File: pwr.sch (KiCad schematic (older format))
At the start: 12 parts, among them J6 Conn_01x02, Q2 FDC6420C, U5 SGM2036_UTDFN, U7 SGM40561

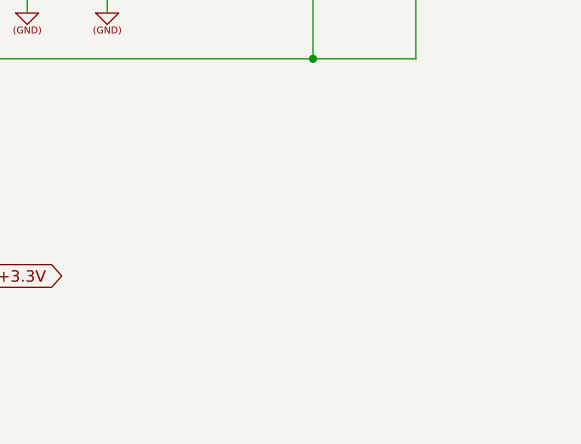
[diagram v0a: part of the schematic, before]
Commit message: Build power board
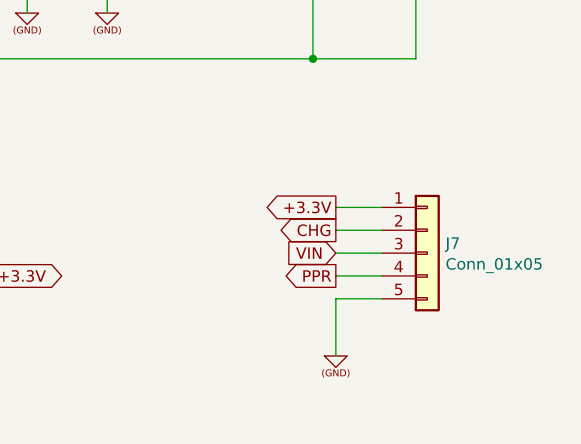
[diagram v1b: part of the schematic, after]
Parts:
- added J7: Conn_01x05, Pin_Headers:Pin_Header_Straight_1x05_Pitch2.54mm, symbol Connector_Generic:Conn_01x05
- Q2: footprint TO_SOT_Packages_SMD:SOT-666 -> TO_SOT_Packages_SMD:SuperSOT-6
- U5: footprint (none) -> TO_SOT_Packages_SMD:SOT-23-5
- U7: footprint Housings_DFN_QFN:VDFN-8-1EP_2x2mm_Pitch0.5mm -> Housings_DFN_QFN:TDFN-2x2-8L
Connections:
- wire segments 56 -> 62
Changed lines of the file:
@@
 F 0 "U7" H 4350 4600 50  0000 C CNN
 F 1 "SGM40561" H 5050 4550 50  0000 C CNN
-F 2 "Housings_DFN_QFN:VDFN-8-1EP_2x2mm_Pitch0.5mm" H 4650 4100 50  0001 C CNN
+F 2 "Housings_DFN_QFN:TDFN-2x2-8L" H 4650 4100 50  0001 C CNN
 F 3 "" H 4650 4100 50  0001 C CNN
 	1    4650 4100
@@
 F 0 "U5" H 4600 6582 50  0000 C CNN
 F 1 "SGM2036_UTDFN" H 4600 6491 50  0000 C CNN
-F 2 "" H 4600 6050 50  0001 C CNN
+F 2 "TO_SOT_Packages_SMD:SOT-23-5" H 4600 6050 50  0001 C CNN
 F 3 "" H 4600 6050 50  0001 C CNN
 	1    4600 6050
@@
 F 0 "Q2" V 7178 3900 50  0000 C CNN
 F 1 "FDC6420C" V 7087 3900 50  0000 C CNN
-F 2 "TO_SOT_Packages_SMD:SOT-666" H 7050 3825 50  0001 L CNN
+F 2 "TO_SOT_Packages_SMD:SuperSOT-6" H 7050 3825 50  0001 L CNN
 F 3 "http://www.irf.com/product-info/datasheets/data/irf7309ipbf.pdf" H 6850 3900 50  0001 L CNN
 	2    6850 3900
@@
 Wire Wire Line
 	4100 3100 4550 3100
+Text GLabel 6950 5650 0    50   Input ~ 0
+VIN
+$Comp
+L power:(GND) #PWR024
+U 1 1 5DA84AA6
+P 6950 6100
+F 0 "#PWR024" H 6950 6100 30  0001 C CNN
+F 1 "(GND)" H 6950 6100 30  0001 C CNN
+F 2 "" H 6950 6100 60  0000 C CNN
+F 3 "" H 6950 6100 60  0000 C CNN
+	1    6950 6100
+	1    0    0    -1
+$EndComp
+Text GLabel 6950 5450 0    50   Output ~ 0
++3.3V
+Text GLabel 6950 5550 0    50   Output ~ 0
+CHG
+Text GLabel 6950 5750 0    50   Output ~ 0
+PPR
+$Comp
+L Connector_Generic:Conn_01x05 J7
+U 1 1 5DA87273
+P 7350 5650
+F 0 "J7" H 7430 5692 50  0000 L CNN
+F 1 "Conn_01x05" H 7430 5601 50  0000 L CNN
+F 2 "Pin_Headers:Pin_Header_Straight_1x05_Pitch2.54mm" H 7350 5650 50  0001 C CNN
+F 3 "~" H 7350 5650 50  0001 C CNN
+	1    7350 5650
+	1    0    0    -1
+$EndComp
+Wire Wire Line
+	7150 5850 6950 5850
+Wire Wire Line
+	6950 5850 6950 6100
+Wire Wire Line
+	7150 5750 6950 5750
+Wire Wire Line
+	7150 5650 6950 5650
+Wire Wire Line
+	7150 5550 6950 5550
+Wire Wire Line
+	7150 5450 6950 5450
 $EndSCHEMATC

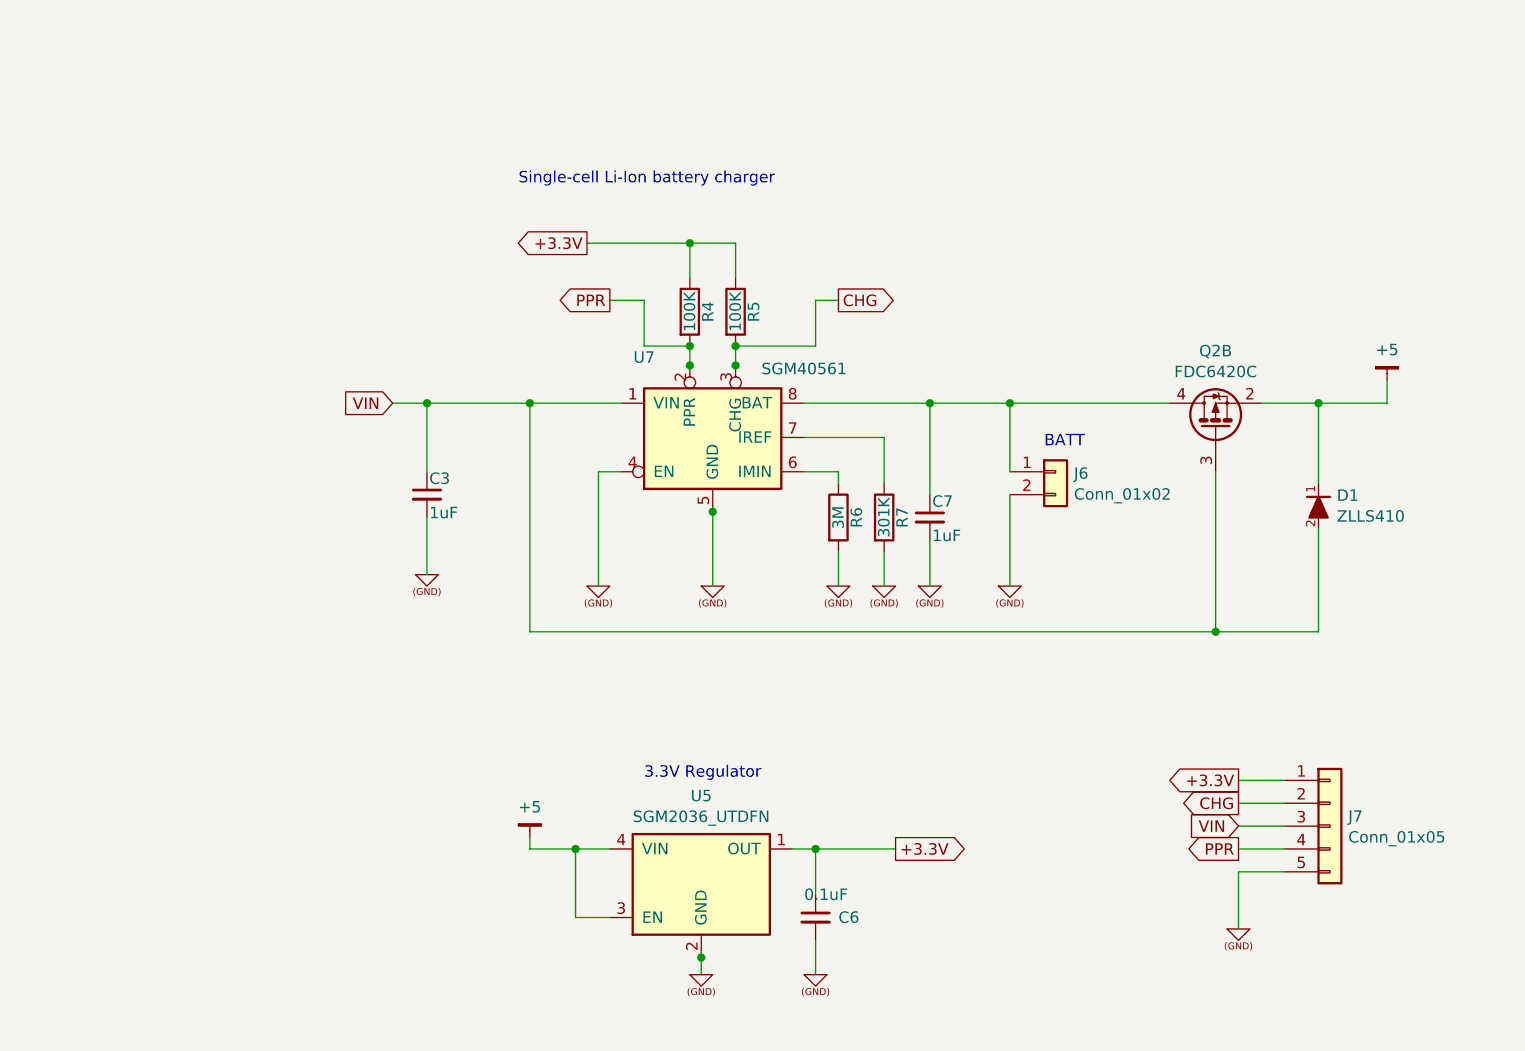
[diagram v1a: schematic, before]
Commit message: v.01 power board PCB
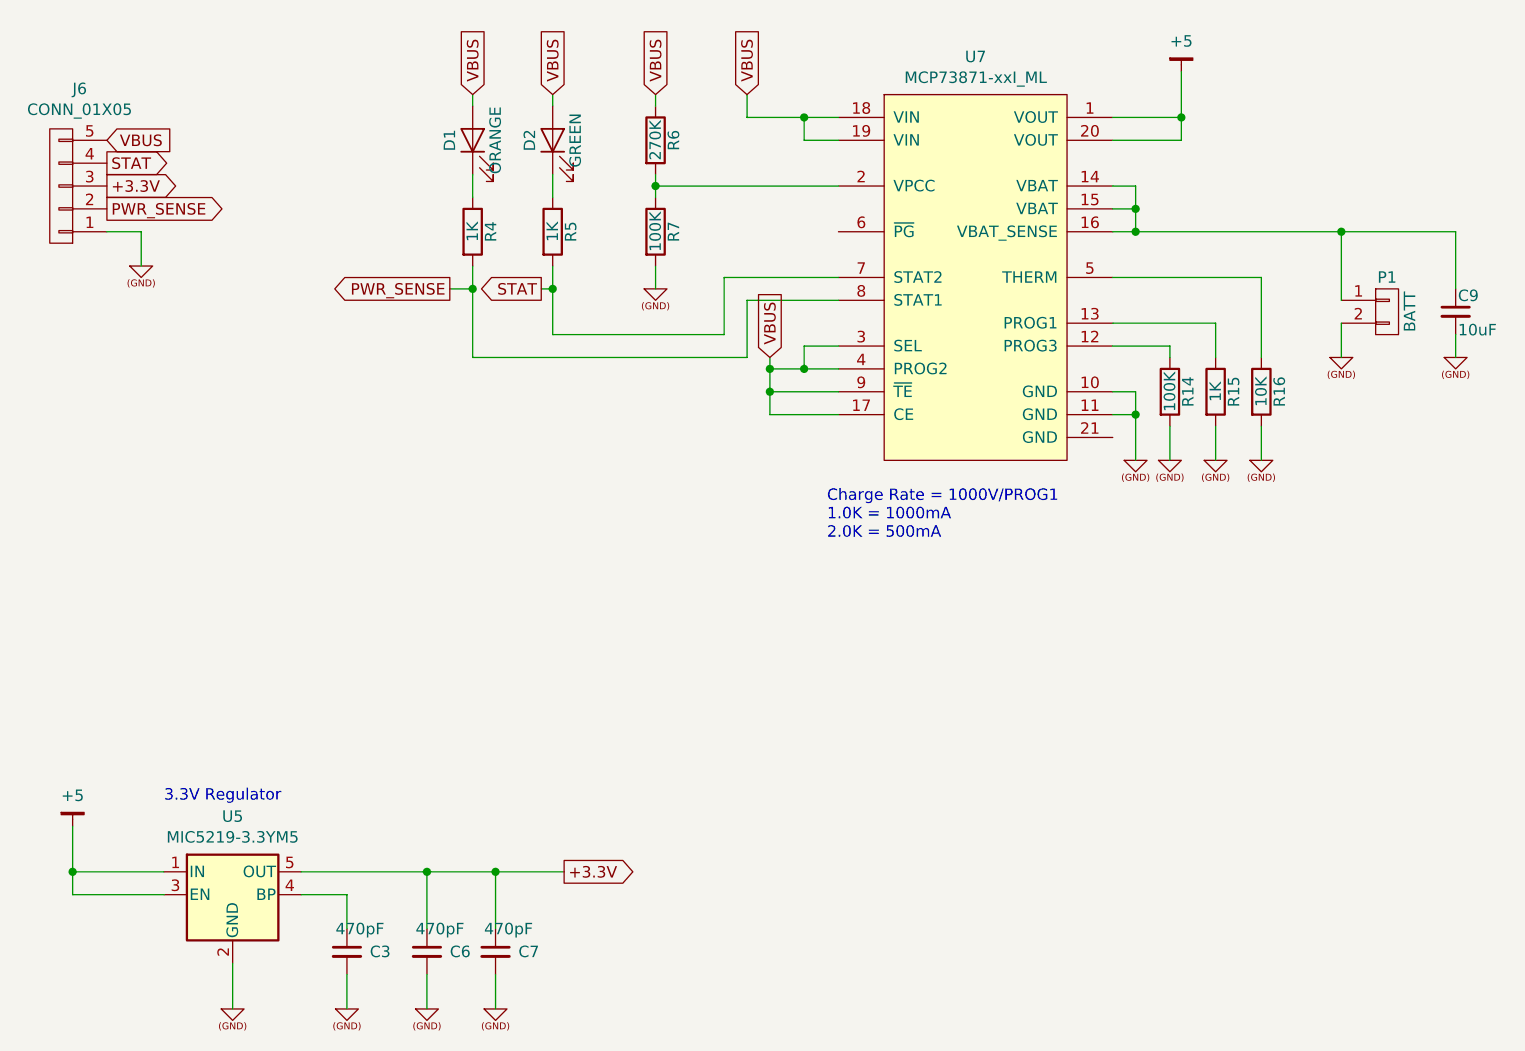
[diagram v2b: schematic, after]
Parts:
- removed D1: ZLLS410, Diodes_SMD:D_SOD-323, symbol _semi:DIODE
- removed J6: Conn_01x02, my-fp-library:Battery Pads 3x3, symbol Connector_Generic:Conn_01x02
- removed J7: Conn_01x05, Pin_Headers:Pin_Header_Straight_1x05_Pitch2.54mm, symbol Connector_Generic:Conn_01x05
- removed Q2: FDC6420C, TO_SOT_Packages_SMD:SuperSOT-6, symbol mosfet:FDC6420C
- removed U5: SGM2036_UTDFN, TO_SOT_Packages_SMD:SOT-23-5, symbol Power_Management:SGM2036_UTDFN
- removed U7: SGM40561, Housings_DFN_QFN:TDFN-2x2-8L, symbol Power_Management:SGM40561
- added C9: 10uF, Capacitors_SMD:C_0805_HandSoldering, symbol Device:C_Small
- added D1: ORANGE, LEDs:LED_0805, symbol Device:LED
- added D2: GREEN, LEDs:LED_0805, symbol Device:LED
- added J6: CONN_01X05, Pin_Headers:Pin_Header_Straight_1x05_Pitch1.27mm, symbol nrf-rescue:CONN_01X05-conn
- added P1: BATT, my-fp-library:Battery Pads 3x3, symbol nrf-rescue:CONN_01X02-conn
- added R14: 100K, Resistors_SMD:R_0805_HandSoldering, symbol Device:R
- added R15: 1K, Resistors_SMD:R_0805_HandSoldering, symbol Device:R
- added R16: 10K, Resistors_SMD:R_0805_HandSoldering, symbol Device:R
- added U5: MIC5219-3.3YM5, TO_SOT_Packages_SMD:SOT-23-5, symbol Regulator_Linear:MIC5219-3.3YM5
- added U7: MCP73871-xxI_ML, Housings_DFN_QFN:QFN-20-1EP_4x4mm_Pitch0.5mm, symbol nrf-rescue:MCP73871-xxI_ML-microchip
- C3, C7: value 1uF -> 470pF
- C6: value 0.1uF -> 470pF
- R4, R5: value 100K -> 1K; footprint Resistors_SMD:R_0805 -> Resistors_SMD:R_0805_HandSoldering
- R6: value 3M -> 270K; footprint Resistors_SMD:R_0805 -> Resistors_SMD:R_0805_HandSoldering
- R7: value 301K -> 100K; footprint Resistors_SMD:R_0805 -> Resistors_SMD:R_0805_HandSoldering
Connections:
- net labels added: PWR_SENSE, STAT, VBUS
- net labels removed: CHG, PPR, VIN
- wire segments 62 -> 80
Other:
- note added: "Charge Rate = 1000V/PROG1\n1.0K = 1000mA\n2.0K = 500mA"
- note removed: "BATT"
- note removed: "Single-cell Li-Ion battery charger"
